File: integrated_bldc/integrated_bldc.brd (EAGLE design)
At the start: 26.1 x 22.8 mm, 70 parts, among them J2 PRG

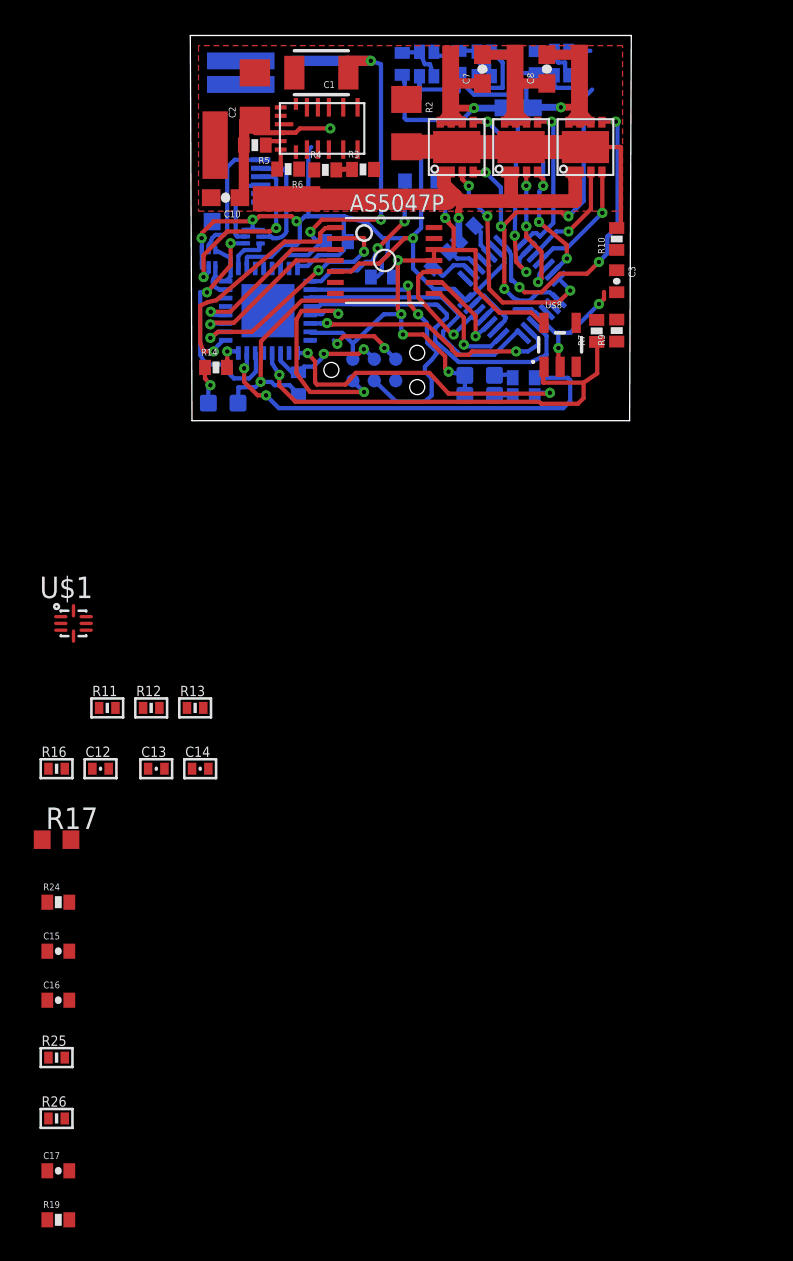
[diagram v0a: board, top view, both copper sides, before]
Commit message: Working on layout.
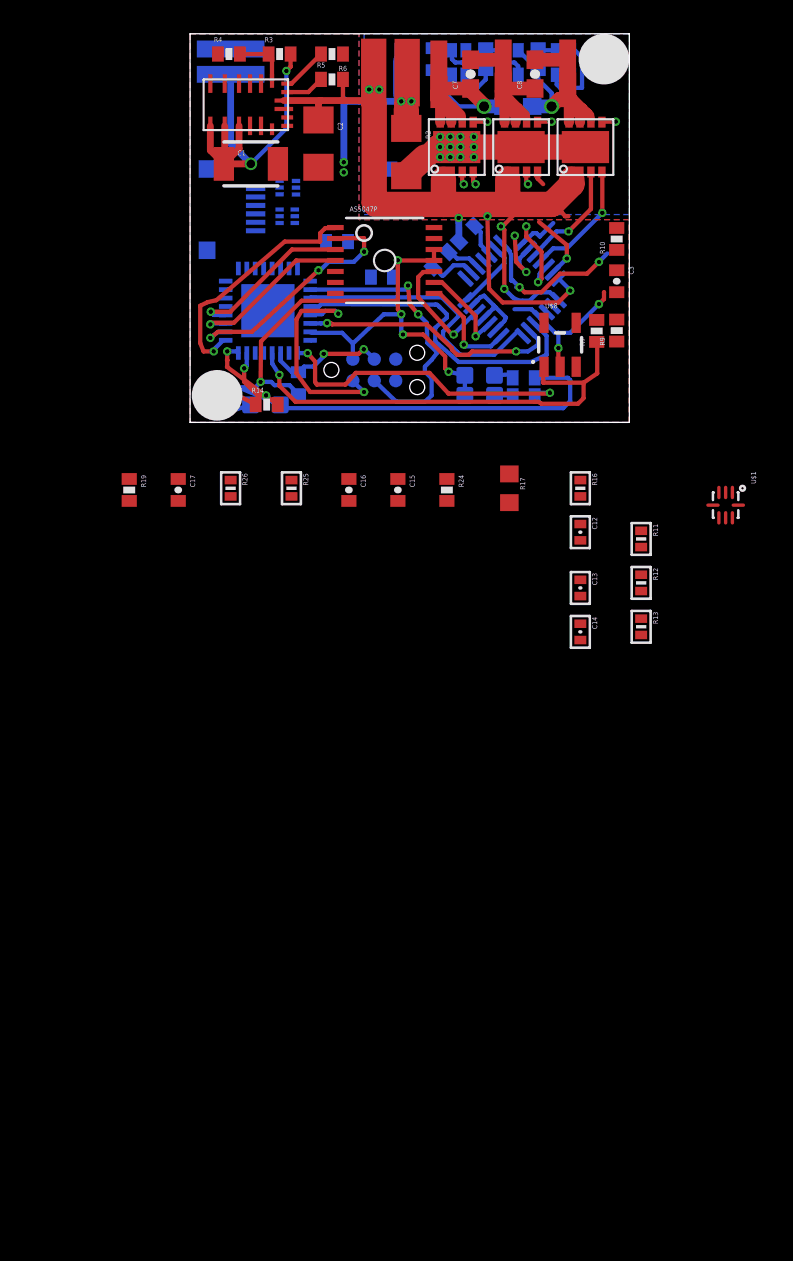
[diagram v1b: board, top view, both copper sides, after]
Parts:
- SJ1, SJ2, SJ3, SJ4: device dhaldane:SJ_TINY -> modular_robotics:SJ_TINY
- moved R19 43.4 mm to (-3.60, -4.00), turned to 270 degrees
- moved C17 40.9 mm to (-0.70, -4.00), turned to 270 degrees
- moved U$1 39.2 mm to (31.7, -4.90), turned to 270 degrees
- moved R26 38.7 mm to (2.40, -3.90), turned to 270 degrees
- moved R25 36.5 mm to (6.00, -3.90), turned to 270 degrees
- moved R16 35.2 mm to (23.1, -3.90), turned to 270 degrees
- moved C16 34.8 mm to (9.40, -4.00), turned to 270 degrees
- moved R17 33.9 mm to (18.9, -3.90), turned to 270 degrees
- moved C15 33.9 mm to (12.3, -4.00), turned to 270 degrees
- moved R24 33.5 mm to (15.2, -4.00), turned to 270 degrees
- moved R11 33.1 mm to (26.7, -6.90), turned to 270 degrees
- moved C12 31.7 mm to (23.1, -6.50), turned to 270 degrees
- moved R12 29.9 mm to (26.7, -9.50), turned to 270 degrees
- moved C13 27.3 mm to (23.1, -9.80), turned to 270 degrees
- moved R13 26.8 mm to (26.7, -12.1), turned to 270 degrees
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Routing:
- net GND: track 69.1 -> 28.0 mm, vias 8 -> 6
- net TB: track 26.2 -> 10.0 mm, vias 3 -> 1
- net I2C_SCL: track 14.0 -> 0.00 mm, vias 2 -> 0
- net TA: track 30.3 -> 17.7 mm, vias 4 -> 3
- net +3V3: track 51.3 -> 39.6 mm, vias 6 -> 5
- net N$38: track 10.9 -> 0.00 mm, vias 2 -> 0
- net TEMP: track 9.67 -> 0.00 mm, vias 2 -> 0
- net GLC: track 18.5 -> 10.4 mm
- net N$36: track 7.78 -> 0.00 mm
- net GLA: track 12.5 -> 5.03 mm
- net N$37: track 6.81 -> 0.00 mm
- net MOTGND: track 17.7 -> 11.6 mm, vias 0 -> 3
- net GLB: track 9.34 -> 3.30 mm
- net N$39: track 4.68 -> 0.00 mm
- net N$10: track 2.33 -> 6.87 mm
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- added copper zone on layer 16, net GND
- added copper zone on layer 16, net MOTGND
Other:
- board size 26.1 x 22.8 mm -> 26 x 23 mm
